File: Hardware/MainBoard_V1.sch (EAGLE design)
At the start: 25 parts, among them IC1 REG1117, J1 NANO_FOOTPRINTNANO, J4 I2C, K1 RELAY-SPDT-JZC-11F, Q2 600mA/40V, Q3 600mA/40V, U1 MOC3021M, U2 TXB0104, U4 MCT2EM, X2 AC

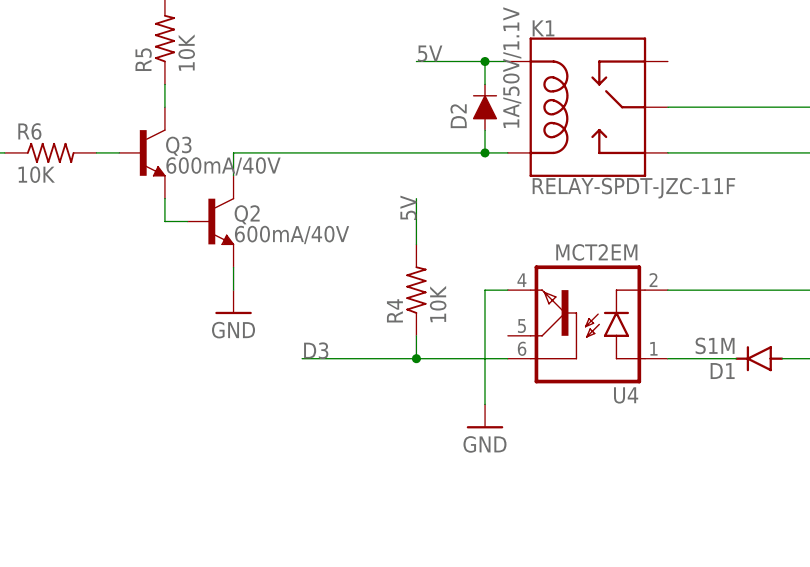
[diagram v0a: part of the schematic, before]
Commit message: Bug fix
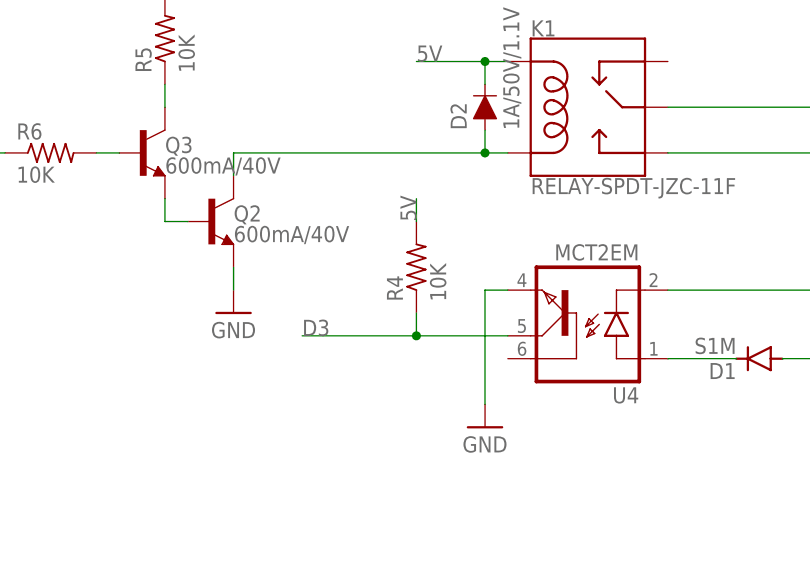
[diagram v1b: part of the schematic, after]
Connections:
- net D3: now also U4.COL; no longer U4.BAS
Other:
- moved on the sheet: R4
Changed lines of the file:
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@@
 <attribute name="VALUE" x="160.02" y="107.315" size="1.778" layer="96" align="center"/>
 </instance>
-<instance part="R4" gate="G$1" x="152.4" y="124.46" smashed="yes" rot="R90">
-<attribute name="NAME" x="150.9014" y="120.65" size="1.778" layer="95" rot="R90"/>
-<attribute name="VALUE" x="155.702" y="120.65" size="1.778" layer="96" rot="R90"/>
+<instance part="R4" gate="G$1" x="152.4" y="127" smashed="yes" rot="R90">
+<attribute name="NAME" x="150.9014" y="123.19" size="1.778" layer="95" rot="R90"/>
+<attribute name="VALUE" x="155.702" y="123.19" size="1.778" layer="96" rot="R90"/>
 </instance>
 <instance part="Q2" gate="G$1" x="129.54" y="132.08" smashed="yes">
@@
 <segment>
 <pinref part="R4" gate="G$1" pin="2"/>
-<wire x1="152.4" y1="129.54" x2="152.4" y2="134.62" width="0.1524" layer="91"/>
+<wire x1="152.4" y1="132.08" x2="152.4" y2="134.62" width="0.1524" layer="91"/>
 <label x="152.4" y="132.08" size="1.778" layer="95" rot="R90"/>
 </segment>
@@
 </segment>
 <segment>
-<pinref part="U4" gate="A" pin="BAS"/>
-<wire x1="162.56" y1="116.84" x2="152.4" y2="116.84" width="0.1524" layer="91"/>
 <pinref part="R4" gate="G$1" pin="1"/>
-<wire x1="152.4" y1="116.84" x2="139.7" y2="116.84" width="0.1524" layer="91"/>
-<wire x1="152.4" y1="119.38" x2="152.4" y2="116.84" width="0.1524" layer="91"/>
-<junction x="152.4" y="116.84"/>
-<label x="139.7" y="116.84" size="1.778" layer="95"/>
-</segment>
-</net>
+<wire x1="152.4" y1="119.38" x2="139.7" y2="119.38" width="0.1524" layer="91"/>
+<wire x1="152.4" y1="121.92" x2="152.4" y2="119.38" width="0.1524" layer="91"/>
+<label x="139.7" y="119.38" size="1.778" layer="95"/>
+<pinref part="U4" gate="A" pin="COL"/>
+<wire x1="162.56" y1="119.38" x2="152.4" y2="119.38" width="0.1524" layer="91"/>
+<junction x="152.4" y="119.38"/>
+</segment>
+</net>
